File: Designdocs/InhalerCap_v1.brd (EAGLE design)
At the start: 23.8 x 23.6 mm, 5 parts

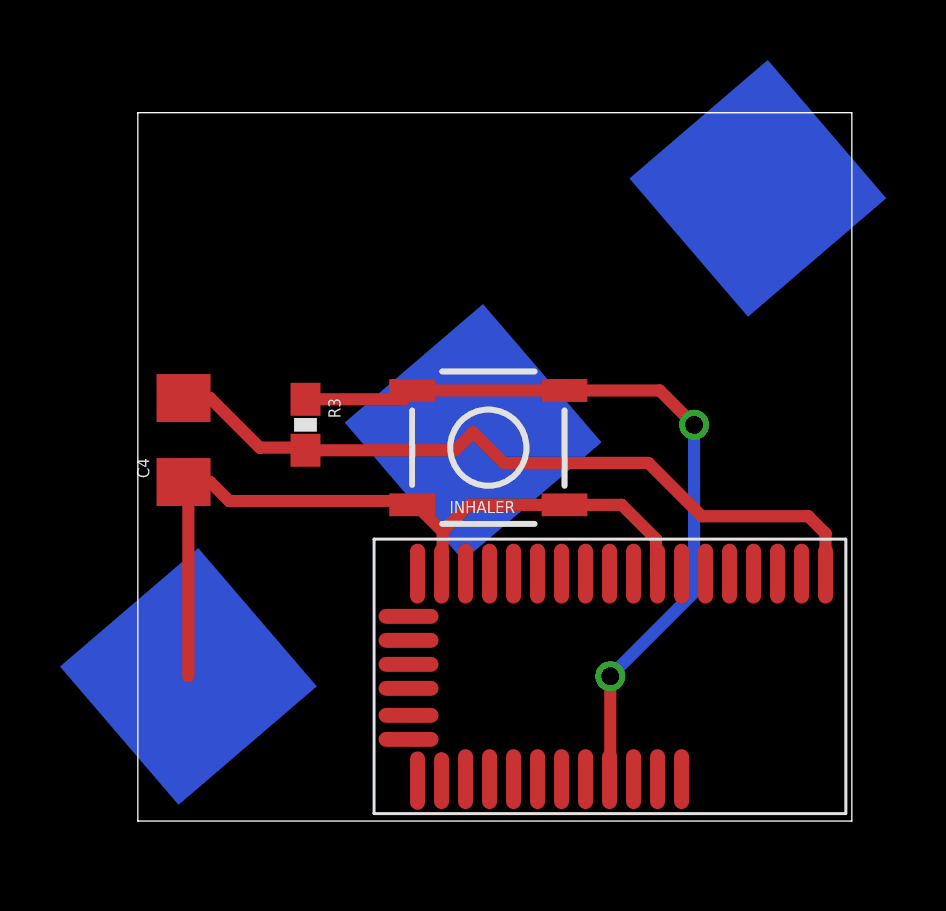
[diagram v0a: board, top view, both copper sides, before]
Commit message: Updated documentation
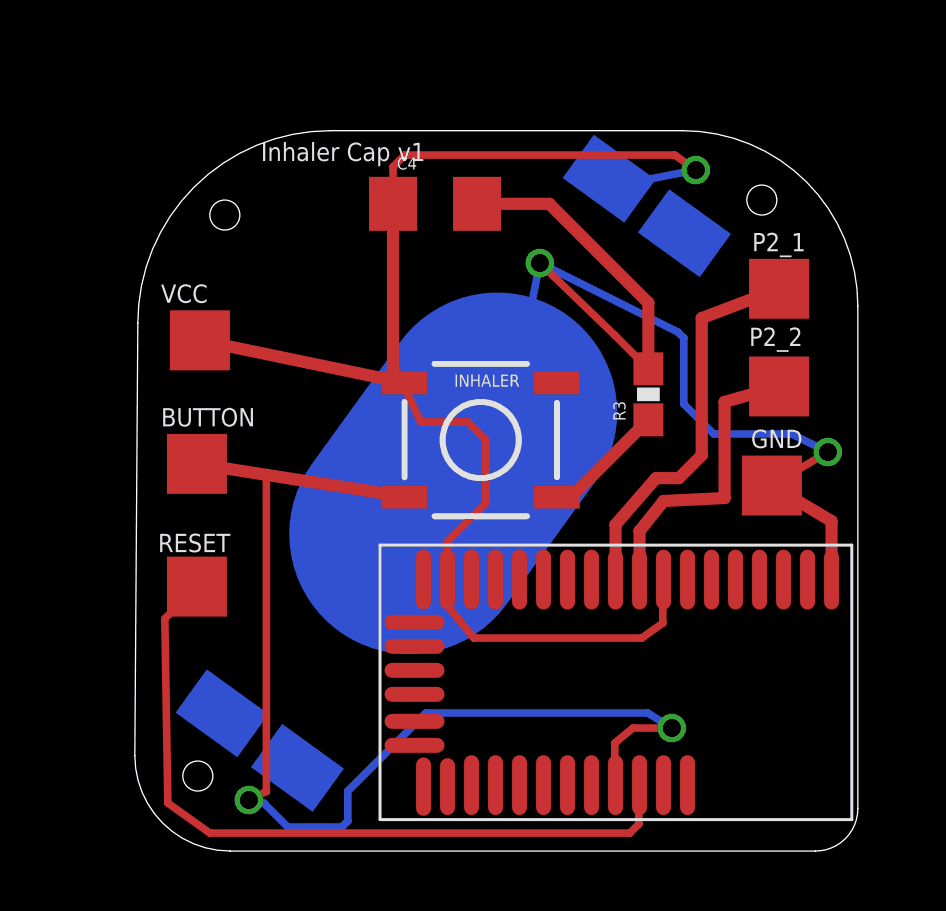
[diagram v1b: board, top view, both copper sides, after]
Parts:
- removed BAT1: 3V, SparkFun-Electromechanical:BATTCON_20MM
- added BAT2: 20mm coincell, SparkFun-Electromechanical:BATTCON_20MM_4LEGS
- added BUTTON, GND, P2_1, P2_2, RESET, VCC: TPTP20SQ, testpad:TP20SQ
- moved C4 11.5 mm to (9.91, 20.6), turned to 0 degrees
- moved R3 11.5 mm to (17.0, 14.2), turned to 90 degrees
- moved INHALER 0.36 mm to (11.4, 12.7), turned to 0 degrees
- moved U$1 0.28 mm to (8.07, 9.20)
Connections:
- new net 1: INHALER.4, R3.1
- new net P2_1: P2_1.TP, U$1.P2_1
- new net P2_2: P2_2.TP, U$1.P2_2
- new net RESET: RESET.TP, U$1.RESET#
- net BUTTON: now also BUTTON.TP; no longer INHALER.4, R3.1
- net GND: now also BAT2.2, GND.TP; no longer BAT1.2
- net VCC: now also BAT2.1, VCC.TP; no longer BAT1.1, INHALER.2
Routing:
- net RESET: track 0.00 -> 25.1 mm
- net VCC: track 26.5 -> 46.9 mm, vias 0 -> 1
- net GND: track 25.1 -> 44.6 mm, vias 0 -> 2
- net P2_1: track 0.00 -> 13.1 mm
- net BUTTON: track 26.5 -> 38.6 mm
- net P2_2: track 0.00 -> 10.0 mm
- net 1: track 0.00 -> 4.12 mm
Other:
- board size 23.8 x 23.6 mm -> 24.1 x 24 mm
- board text added: "Inhaler Cap v1"
